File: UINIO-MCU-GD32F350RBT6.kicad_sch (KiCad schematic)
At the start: 33 parts, among them J1 Conn_01x32_Pin, J2 Conn_01x32_Pin, J3 Conn_01x04_Pin, SW1 BOOT0, SW2 NRST, U1 ME6211C33M5G-N, U2 GD32F350RBT6, Y1 32.768KHz, Y2 8MHz

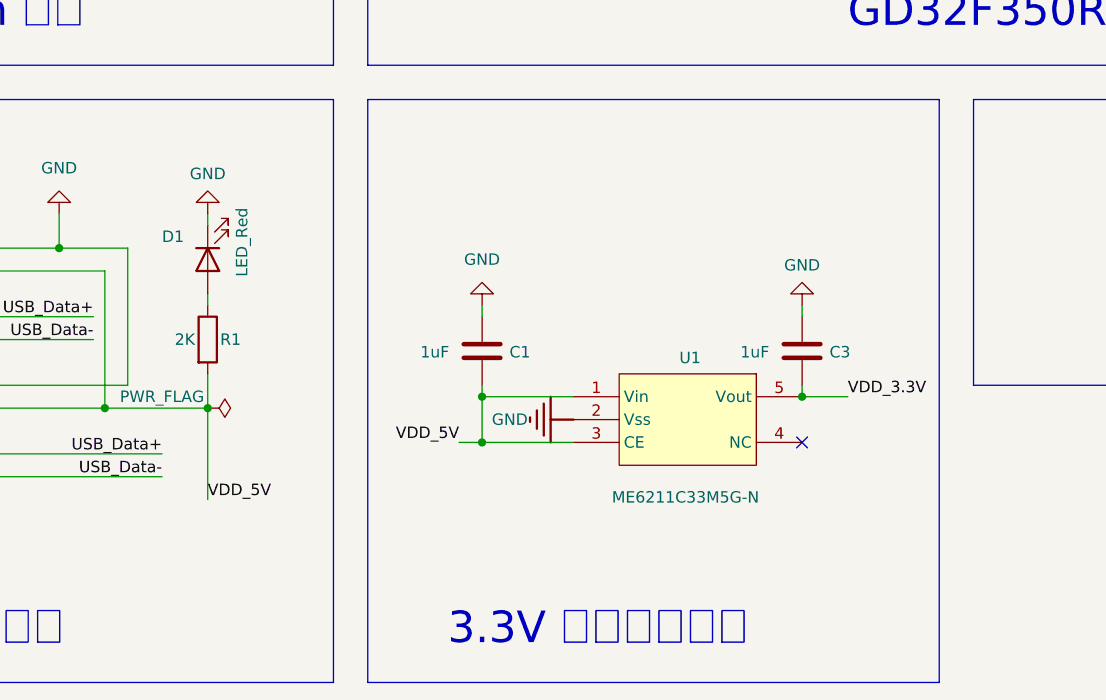
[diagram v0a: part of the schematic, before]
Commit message: Release UINIO-MCU-GD32F350RBT6 version 3.1.1.
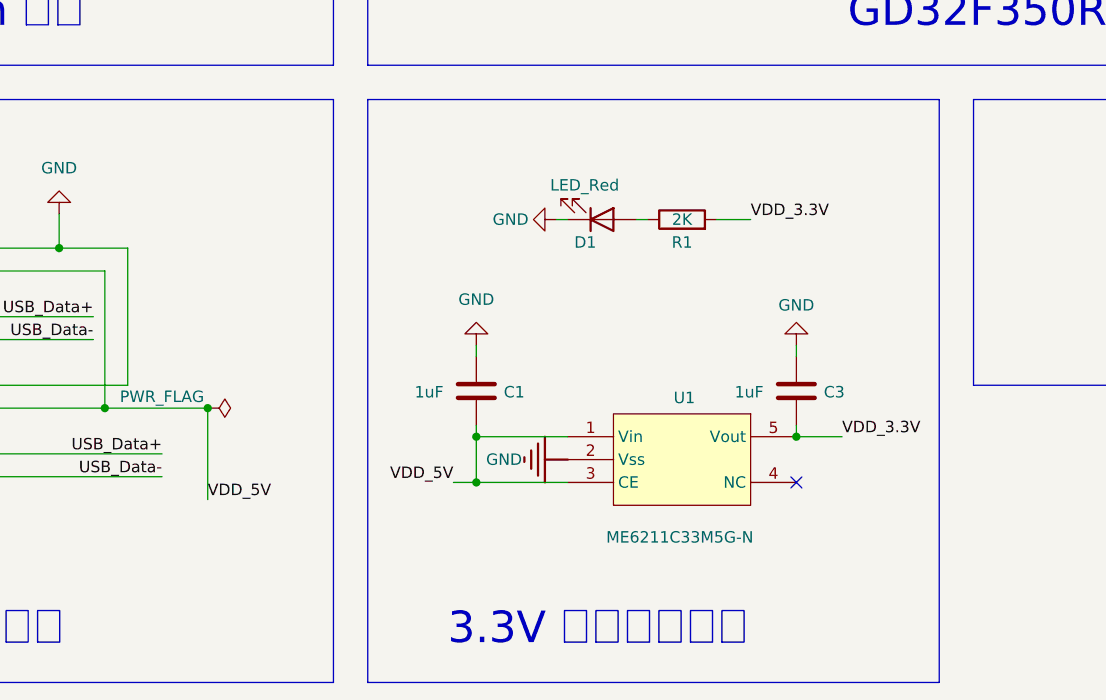
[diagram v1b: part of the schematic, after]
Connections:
- net VDD_3.3V: now also R1.2
- net VDD_5V: no longer R1.2
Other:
- moved on the sheet: C1, C3, D1, R1, U1
